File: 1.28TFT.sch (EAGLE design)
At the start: 12 parts, among them M1 LCD_FPCST

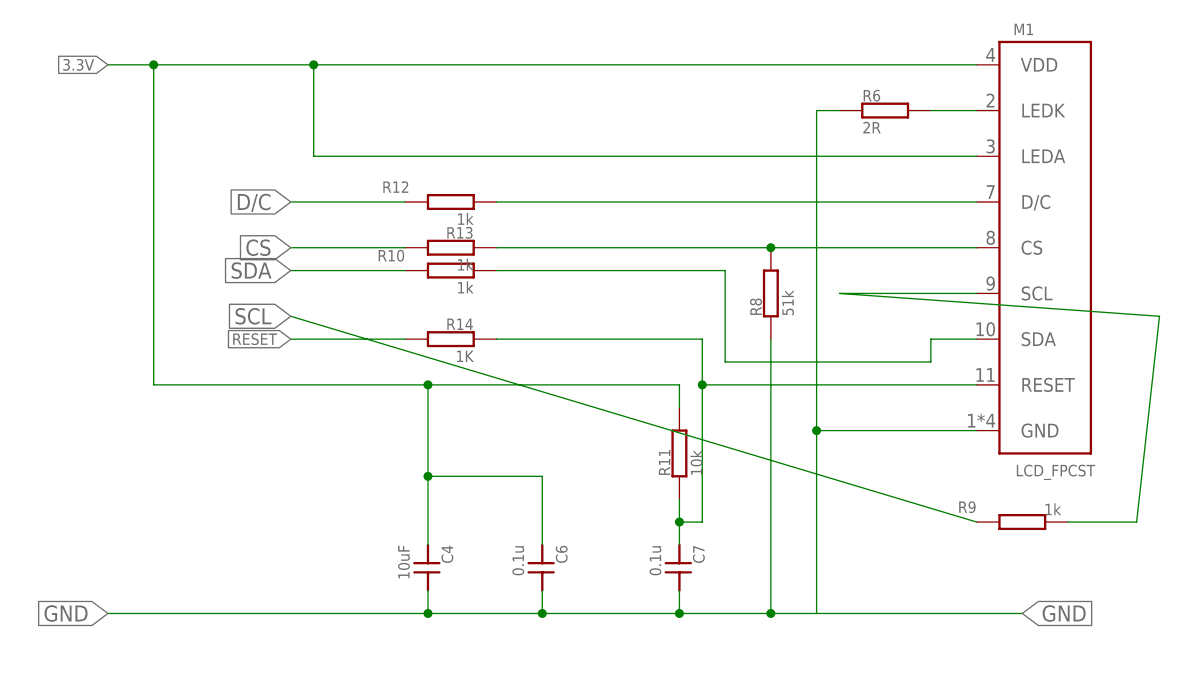
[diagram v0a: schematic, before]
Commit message: bugfix
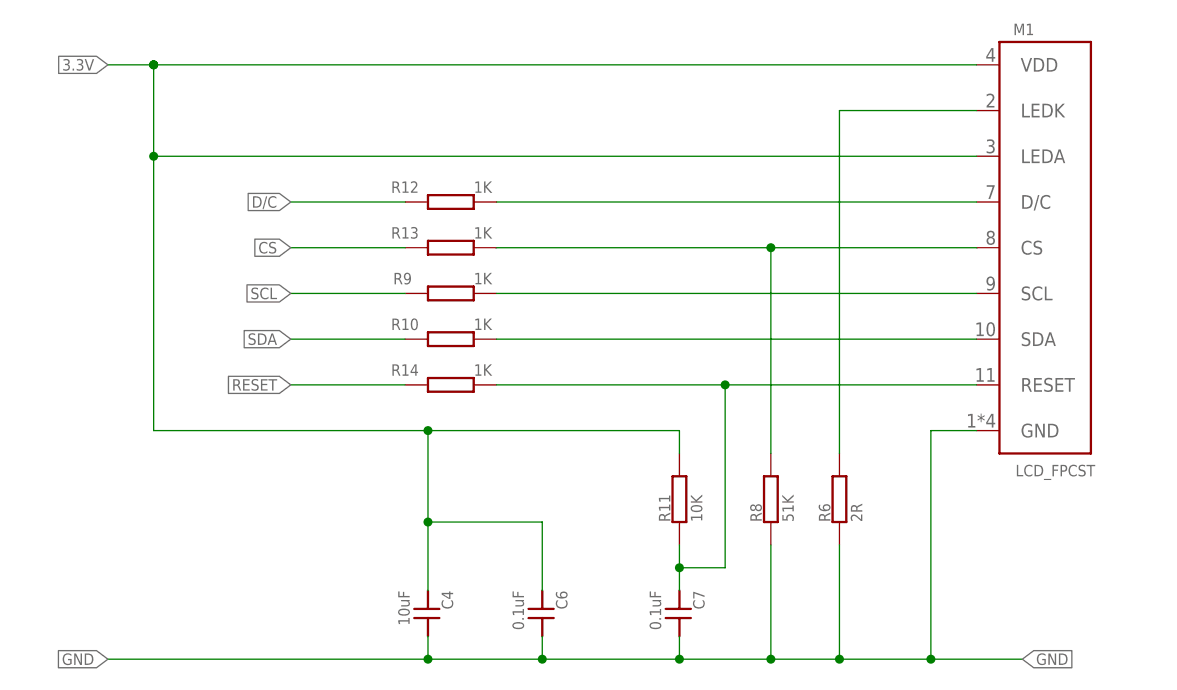
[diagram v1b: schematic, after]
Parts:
- C6, C7: value 0.1u -> 0.1uF
- R10, R12, R13, R9: value 1k -> 1K
- R11: value 10k -> 10K
- R8: value 51k -> 51K
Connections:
- net DC renamed N$5
- new net N$4: M1.SDA, R10.P$1
- net SDA: no longer M1.SDA, R10.P$1
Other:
- moved on the sheet: C4, C6, C7, R10, R11, R14, R6, R8, R9
